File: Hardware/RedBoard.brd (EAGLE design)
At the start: 68.6 x 53.3 mm, 63 parts, among them IC3 LM1117, J2 ICSP, J3 POWER_JACKSUPER_BOMB_DIGITY, Q1 ZXMP6A13FTA, U1 FT231XS, U2 MIC5205, U3 ATMEGA328, Y1 16MHz

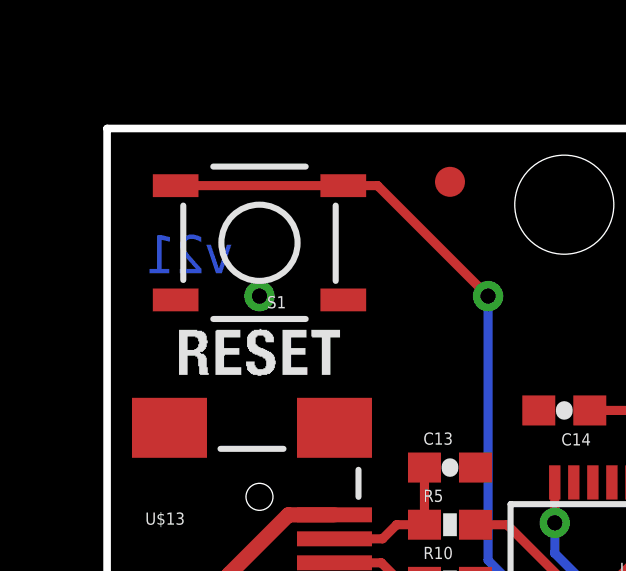
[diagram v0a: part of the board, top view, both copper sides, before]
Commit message: upping version number to v22`
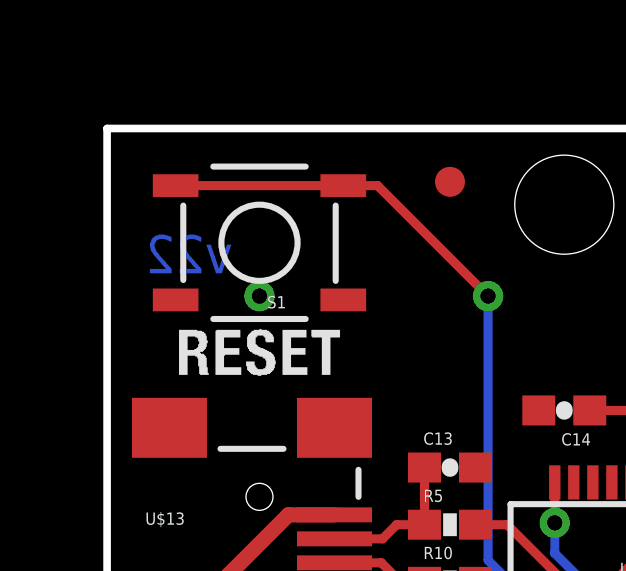
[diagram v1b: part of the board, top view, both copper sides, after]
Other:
- board text added: "v22"
- board text removed: "v21"
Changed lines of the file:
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@@
 <?xml version="1.0" encoding="utf-8"?>
 <!DOCTYPE eagle SYSTEM "eagle.dtd">
-<eagle version="6.5.0">
+<eagle version="6.6.0">
 <drawing>
 <settings>
@@
 <text x="64.77" y="45.593" size="1.4224" layer="26" ratio="12" rot="MR0">MADE IN</text>
 <text x="64.135" y="43.053" size="1.4224" layer="26" ratio="12" rot="MR0">ITALY</text>
-<text x="4.191" y="48.514" size="1.27" layer="16" font="vector" ratio="20" rot="MR0">v21</text>
+<text x="4.191" y="48.514" size="1.27" layer="16" font="vector" ratio="20" rot="MR0">v22</text>
 <text x="32.893" y="-24.13" size="1.778" layer="51" font="vector" ratio="12">J.Lindblom</text>
 <rectangle x1="0.635" y1="22.352" x2="2.032" y2="30.607" layer="43"/>
